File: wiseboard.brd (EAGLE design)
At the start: 80 x 55 mm, 87 parts, among them IC2 LM358MX, Q1 IRLML6402TRPBF, Q2 IRLML6402TRPBF, U1 LT1945EMSPBF, U2 BQ24210DQCT, X1 1528-1438-ND

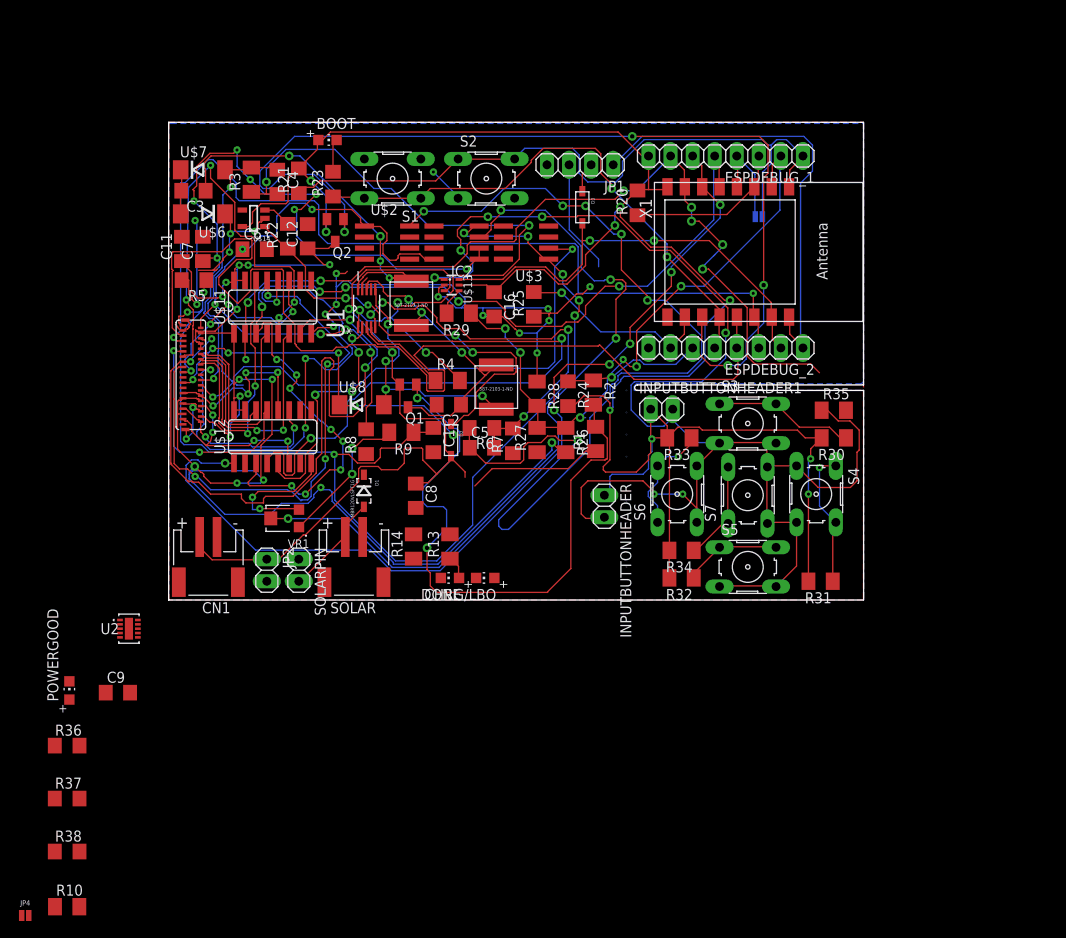
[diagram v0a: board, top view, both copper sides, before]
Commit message: ROUTE REV 1.5 BOARD
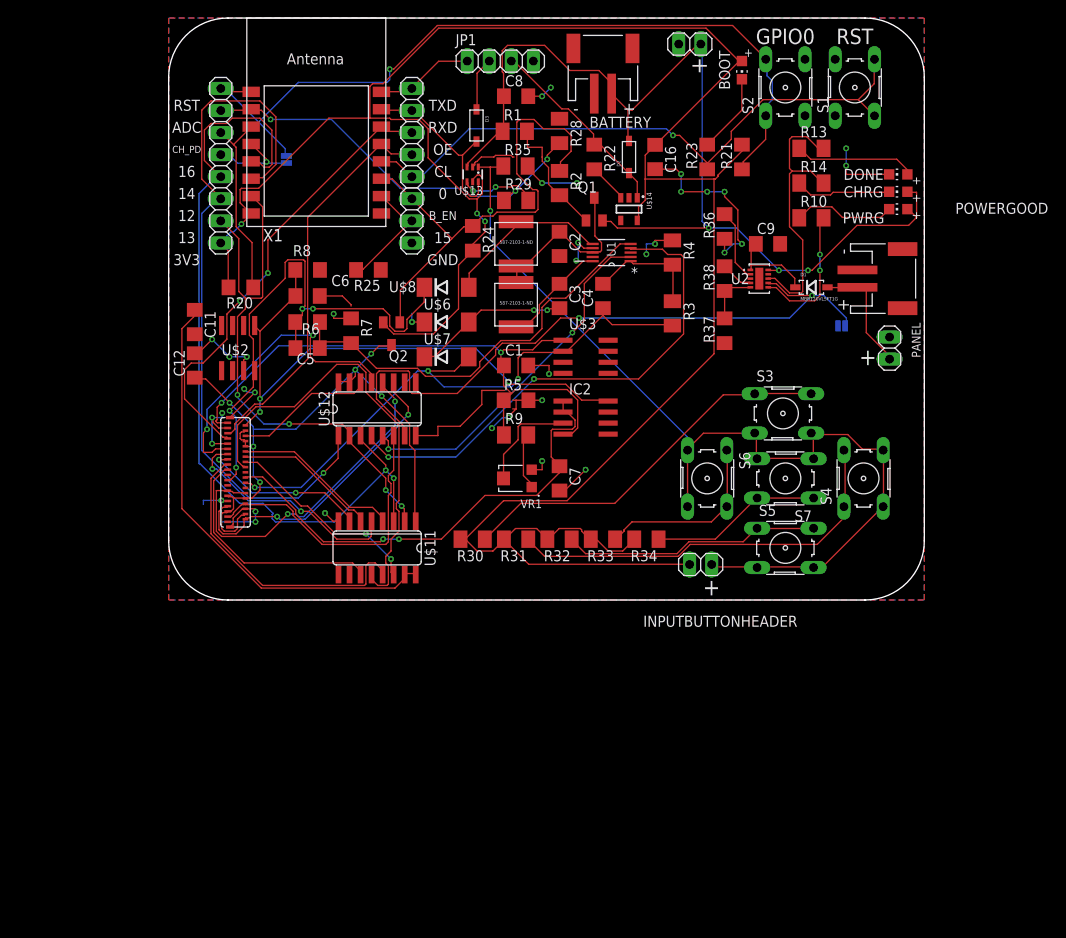
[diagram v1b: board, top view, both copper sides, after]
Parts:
- removed CN1: (no value), adafruit:JST-PH-2-SMT-RA
- removed INPUTBUTTONHEADER1, JP2: (no value), pinhead:1X02
- removed R26: 4K7, adafruit:M1206
- removed R27: 10K, adafruit:M1206
- added BAT_CON: (no value), adafruit:JST-PH-2-SMT-RA
- added BAT_PIN: (no value), pinhead:1X02
- moved R10 116.8 mm to (74.0, 44.0)
- moved JP4 115.9 mm to (77.5, 31.6), flipped to the bottom, turned to 180 degrees
- moved POWERGOOD 110.4 mm to (84.0, 45.0), turned to 90 degrees
- moved R38 100.4 mm to (64.0, 37.0), turned to 90 degrees
- moved R36 96.4 mm to (64.0, 43.0), turned to 90 degrees
- moved R37 92.9 mm to (64.0, 31.0), turned to 90 degrees
- moved C9 90.9 mm to (69.0, 41.0)
- moved U2 83.0 mm to (68.0, 37.0)
- moved SOLARPIN 72.7 mm to (83.0, 29.0)
- moved SOLAR 70.1 mm to (83.0, 37.0), turned to 270 degrees
- moved DONE 69.4 mm to (84.0, 49.0)
- moved CHRG/LBO 65.1 mm to (84.0, 47.0)
- moved R14 62.0 mm to (74.0, 48.0), turned to 0 degrees
- moved R13 61.9 mm to (74.0, 52.0), turned to 0 degrees
- moved ESPDEBUG_1 58.1 mm to (6.00, 50.0), turned to 270 degrees
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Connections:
- removed net N$25: D2.C, R22.1, U$14.1
- new net N$16: C11.1, U$11.15, U$11.16
- net +3V3: no longer INPUTBUTTONHEADER1.1
- net ADC: no longer R26.1, R27.2
- net GND: now also BAT_CON.2, BAT_PIN.2; no longer CN1.2, JP2.2, R27.1
- net N$26: no longer INPUTBUTTONHEADER1.2
- net VBAT: now also BAT_CON.1, BAT_PIN.1; no longer CN1.1, JP2.1
- net VCC: now also D2.C, R22.1, U$14.1
- net VDD: no longer C11.1, R26.2, U$11.15, U$11.16
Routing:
- net VDD: track 178.3 -> 76.8 mm, vias 15 -> 6
- net +22V: track 158.1 -> 61.7 mm, vias 12 -> 4
- net CHARGE_EN: track 0.00 -> 77.8 mm, vias 0 -> 2
- net CL: track 122.3 -> 45.4 mm
- net N$1: track 88.3 -> 12.0 mm, vias 4 -> 0
- net BOOSTENA: track 132.0 -> 57.5 mm, vias 5 -> 0
- net NFB1: track 82.0 -> 13.5 mm, vias 5 -> 0
- net QP3: track 82.8 -> 19.2 mm, vias 4 -> 2
- net N$26: track 173.2 -> 111.2 mm, vias 7 -> 1
- net -15V: track 132.9 -> 71.1 mm, vias 8 -> 2
- net N$3: track 70.9 -> 14.2 mm, vias 2 -> 0
- net N$16: track 0.00 -> 55.3 mm
- net OE: track 105.4 -> 52.2 mm
- net N$25: track 50.3 -> 0.00 mm, vias 4 -> 0
- net TXD: track 52.9 -> 11.3 mm
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- added copper zone on layer 16, net GND
- removed copper zone on layer 16, net N$12
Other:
- board size 80 x 55 mm -> 87 x 67 mm
- board text added: "+"
- board text added: "0"
- board text added: "12"
- board text added: "13"
- board text added: "14"
- board text added: "15"
- board text added: "16"
- board text added: "3V3"
- board text added: "ADC"
- board text added: "BATTERY"
- board text added: "BOOT"
- board text added: "B_EN"
- board text added: "CHRG"
- board text added: "CH_PD"
- board text added: "CL"
- board text added: "DONE"
- board text added: "EN TO GND"
- board text added: "GND"
- board text added: "GPIO0"
- board text added: "OE"
- board text added: "PANEL"
- board text added: "PWRG"
- board text added: "RST"
- board text added: "RST to 16"
- board text added: "RXD"
- board text added: "TXD"
- board text added: "test"
